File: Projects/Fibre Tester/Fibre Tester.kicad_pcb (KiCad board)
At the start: 2 copper layers, 36.5 x 48.2 mm, 8 parts, among them IC1 NE555, J1 JACK-PLUG1

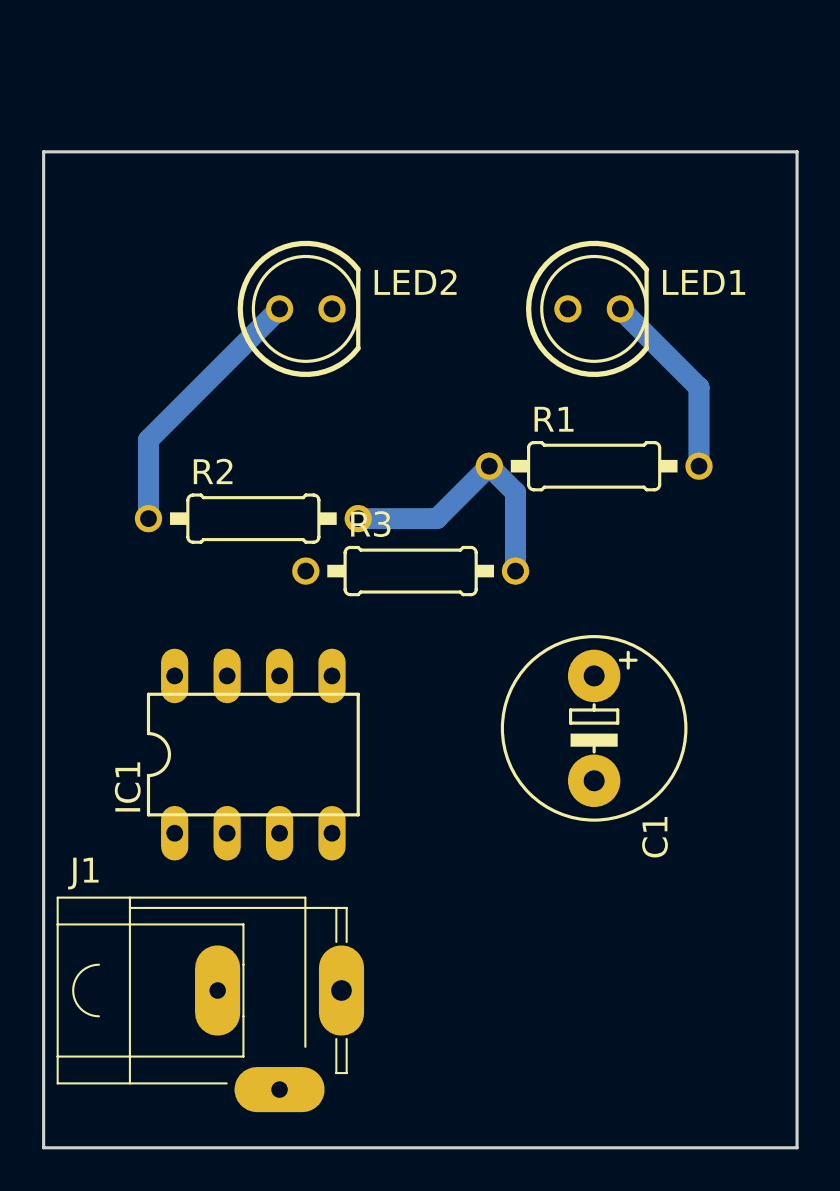
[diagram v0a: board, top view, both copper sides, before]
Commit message: new file:   Libraries/My_Component_Footprints.pretty/Switch_Slide_3_way_pad_SMD.kicad_mod 	modified:   Projects/Fibre Tester/Fibre Tester-cache.lib 	renamed:    Projects/Fibre Tester/Fibre_Tester-eagle-import.dcm -> Projects/Fibre Tester/Fibre Tester-rescue.dcm 	new file:   Projects/Fibre Tester/Fibre Tester-rescue.lib 	new file:   Projects/Fibre Tester/Fibre Tester.bak 	modified:   Projects/Fibre Tester/Fibre Tester.kicad_pcb 	new file:   Projects/Fibre Tester/Fibre Tester.kicad_pcb-bak 	new file:   Projects/Fibre Tester/Fibre Tester.net 	modified:   Projects/Fibre Tester/Fibre Tester.pro 	modified:   Projects/Fibre Tester/Fibre Tester.sch 	deleted:    Projects/Fibre Tester/Fibre_Tester-eagle-import.lib 	new file:   Projects/Fibre Tester/fp-info-cache 	modified:   Projects/Fibre Tester/sym-lib-table
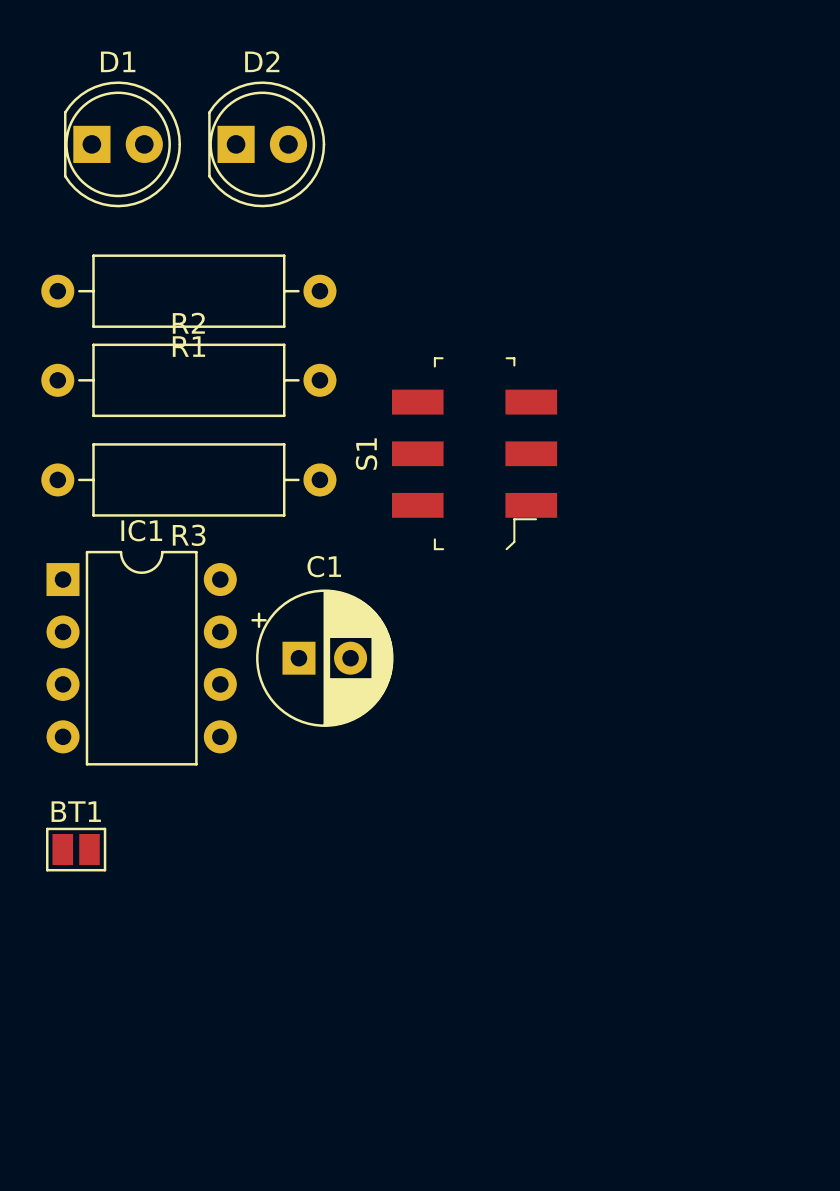
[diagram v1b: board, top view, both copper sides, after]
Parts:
- removed J1: JACK-PLUG1, Fibre Tester:SPC4078
- removed LED1: RED, Fibre Tester:LED5MM
- removed LED2: Green, Fibre Tester:LED5MM
- added BT1: Battery_Cell, Jumper:SolderJumper-2_P1.3mm_Open_Pad1.0x1.5mm, F.Cu at (131.8, 114.7)
- added D1: LED, LED_THT:LED_D5.0mm_Clear, F.Cu at (132.6, 80.5)
- added D2: LED, LED_THT:LED_D5.0mm_Clear, F.Cu at (139.6, 80.5)
- added S1: JS202011SCQN, digikey-footprints:Switch_Slide_JS202011SCQN, F.Cu at (151.1, 95.5)
- C1: value 10uF -> CP; footprint Fibre Tester:E5-8,5 -> Capacitor_THT:CP_Radial_D6.3mm_P2.50mm
- IC1: footprint Fibre Tester:DIL-08 -> Package_DIP:DIP-8_W7.62mm
- R1, R2, R3: footprint Fibre Tester:0207_10 -> Resistor_THT:R_Axial_DIN0309_L9.0mm_D3.2mm_P12.70mm_Horizontal
- moved R1 15.8 mm to (143.6, 87.6), turned to 180 degrees
- moved C1 14.7 mm to (142.6, 105.4), turned to 0 degrees
- moved IC1 12.5 mm to (131.2, 101.6)
- moved R2 11.6 mm to (130.9, 91.9)
- moved R3 6.23 mm to (143.6, 96.8), turned to 180 degrees
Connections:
- net +12V renamed VCC
- IC1 pad 2: Net-(C1-Pad+) -> Net-(C1-Pad1)
- IC1 pad 5: Net-(IC1-Pad5) -> (no net)
- IC1 pad 6: Net-(C1-Pad+) -> Net-(C1-Pad1)
- IC1 pad 7: Net-(IC1-Pad7) -> (no net)
- R3 pad 1: Net-(C1-Pad+) -> Net-(C1-Pad1)
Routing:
- net Net-(IC1-Pad3): track 13.2 -> 0.00 mm
- net Net-(D2-Pad2): track 12.8 -> 0.00 mm
- net Net-(D1-Pad1): track 9.20 -> 0.00 mm
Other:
- board outline removed
- rule pad_to_mask_clearance: 0.2 -> 0
